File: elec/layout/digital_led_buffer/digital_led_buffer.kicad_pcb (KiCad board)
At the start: 2 copper layers, 10 parts

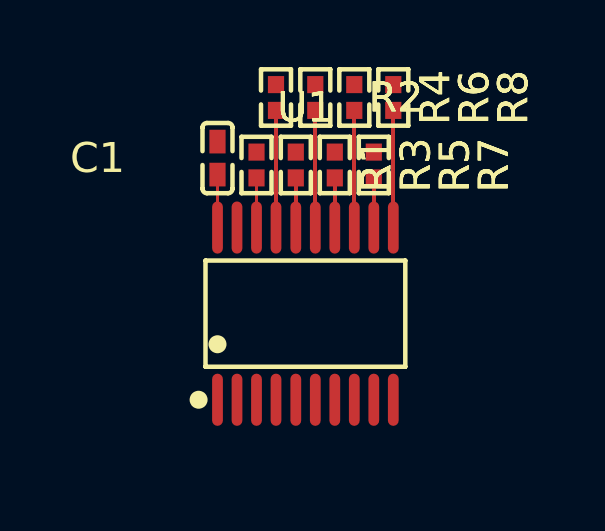
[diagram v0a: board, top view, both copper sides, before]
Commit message: Add pcb files
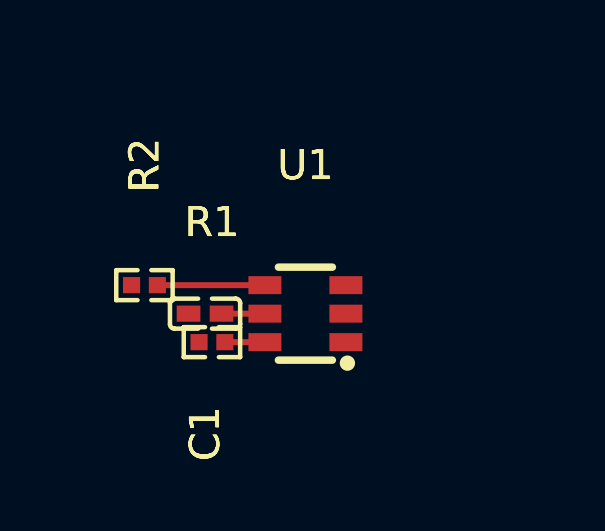
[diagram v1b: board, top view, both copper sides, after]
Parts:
- removed R3, R4, R5, R6, R7, R8: 470Ω ±1% 62.5mW, atopile:R0402-56259e
- U1: footprint atopile:TSSOP-20_L6.5-W4.4-P0.65-LS6.4-BL-86423f -> atopile:SOT-23-6_L2.9-W1.6-P0.95-LS2.8-BR-bfc73b
- moved R2 7.64 mm to (-5.36, -0.95), turned to 0 degrees
- moved R1 6.09 mm to (-3.12, 0.95), turned to 0 degrees
- moved C1 5.20 mm to (-3.35, 0.00), turned to 180 degrees
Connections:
- R1 pad 1: line-18 -> line-5
- R1 pad 2: line-1 -> line-3
- R2 pad 1: line-22 -> line-2
- R2 pad 2: line-2 -> line
- U1 pad 1: hv -> line-1
- U1 pad 2: line-8 -> gnd
- U1 pad 3: line-14 -> line-4
- U1 pad 4: line-19 -> line
- U1 pad 5: line-3 -> hv
- U1 pad 6: line-15 -> line-3
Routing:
- net line: track 0.00 -> 25.1 mm
- net line-5: track 19.6 -> 0.00 mm
- net line-4: track 19.6 -> 0.00 mm
- net line-2: track 19.6 -> 0.00 mm
- net line-13: track 19.6 -> 0.00 mm
- net line-3: track 0.00 -> 9.38 mm
- net line-7: track 8.30 -> 0.00 mm
- net line-20: track 8.30 -> 0.00 mm
- net line-17: track 8.30 -> 0.00 mm
- net line-1: track 8.30 -> 0.00 mm
- net hv: track 8.85 -> 10.1 mm
